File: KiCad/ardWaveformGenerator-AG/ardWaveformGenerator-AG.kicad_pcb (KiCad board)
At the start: 2 copper layers, 97.8 x 55.9 mm, 40 parts, among them SW1 SW_Rotary1x4, U1 Power in, U2 LM386, U3 Output

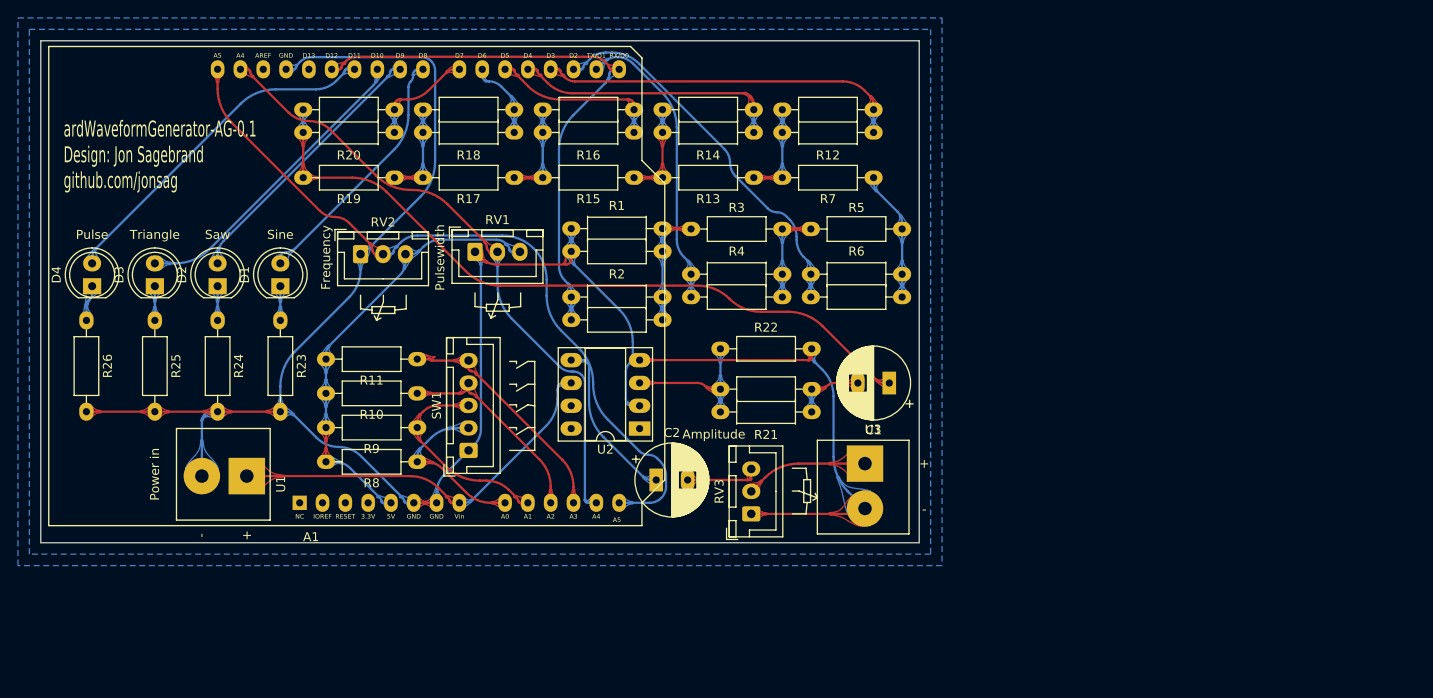
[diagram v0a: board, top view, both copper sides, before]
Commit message: ardWaveformGenerator-AG-pio with pcb-0.2
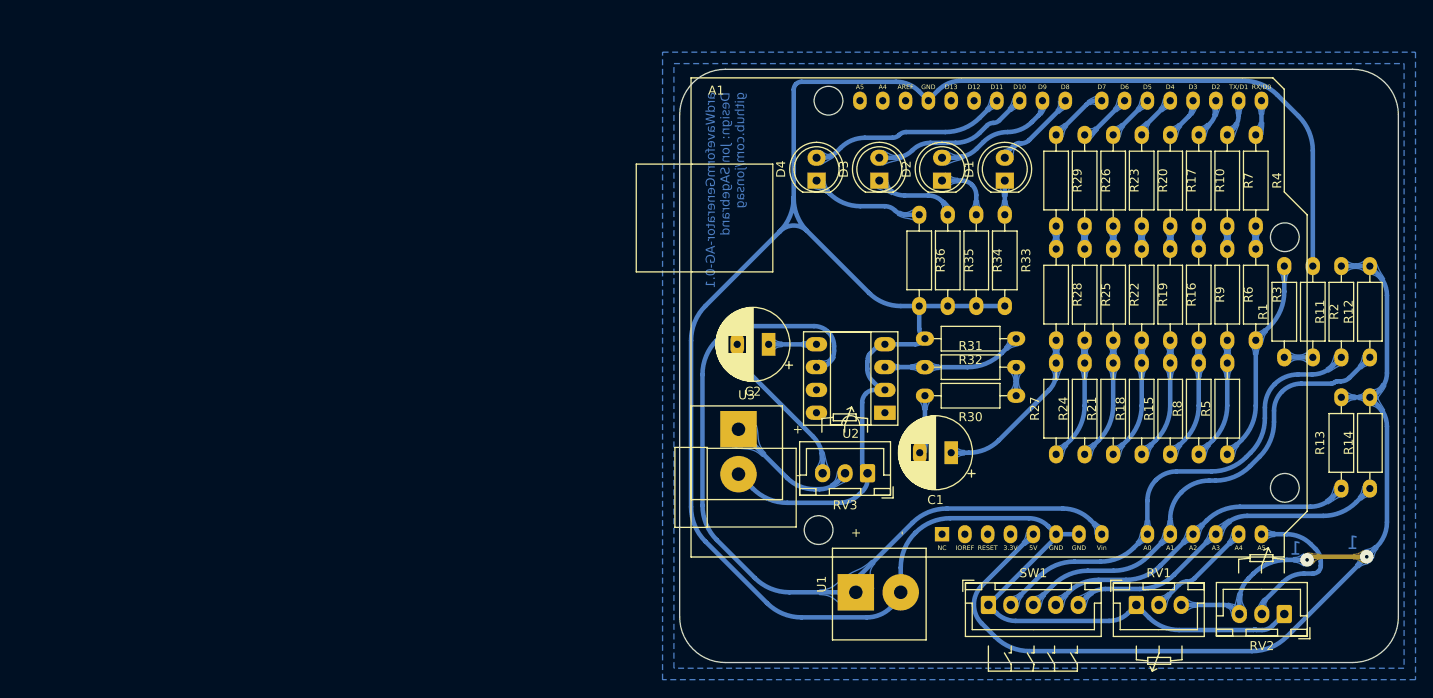
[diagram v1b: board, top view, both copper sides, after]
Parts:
- added R27: 10k, My_Misc:R_Axial_DIN0207_L6.3mm_D2.5mm_P10.16mm_Horizontal_large, F.Cu at (154.9, 107.6)
- added R28: 10k, My_Misc:R_Axial_DIN0207_L6.3mm_D2.5mm_P10.16mm_Horizontal_large, F.Cu at (154.9, 84.8)
- added R29: 10k, My_Misc:R_Axial_DIN0207_L6.3mm_D2.5mm_P10.16mm_Horizontal_large, F.Cu at (154.9, 72.1)
- added R30: 10k, My_Misc:R_Axial_DIN0207_L6.3mm_D2.5mm_P10.16mm_Horizontal_large, F.Cu at (150.5, 101.1)
- added R31: 10k, My_Misc:R_Axial_DIN0207_L6.3mm_D2.5mm_P10.16mm_Horizontal_large, F.Cu at (140.3, 97.9)
- added R32: 2.2k, My_Misc:R_Axial_DIN0207_L6.3mm_D2.5mm_P10.16mm_Horizontal_large, F.Cu at (150.5, 94.8)
- added R33: 220R, My_Misc:R_Axial_DIN0207_L6.3mm_D2.5mm_P10.16mm_Horizontal_large, F.Cu at (149.2, 81.0)
- added R34: 220R, My_Misc:R_Axial_DIN0207_L6.3mm_D2.5mm_P10.16mm_Horizontal_large, F.Cu at (146.1, 81.0)
- added R35: 220R, My_Misc:R_Axial_DIN0207_L6.3mm_D2.5mm_P10.16mm_Horizontal_large, F.Cu at (142.9, 81.0)
- added R36: 220R, My_Misc:R_Axial_DIN0207_L6.3mm_D2.5mm_P10.16mm_Horizontal_large, F.Cu at (139.7, 81.0)
- R1, R12, R14, R16, R18, R2, R20, R21, R4, R6: value 20k -> 10k; footprint My_Parts:R_Axial_parallell_DIN0207_L6.3mm_D2.5mm_P10.16mm_Horizontal_large -> My_Misc:R_Axial_DIN0207_L6.3mm_D2.5mm_P10.16mm_Horizontal_large
- R22: value 2.2k -> 10k
- R23, R24, R25, R26: value 220R -> 10k
- moved R26 113.0 mm to (158.1, 72.1)
- moved RV2 110.4 mm to (180.3, 125.4), turned to 180 degrees
- moved R25 103.8 mm to (158.1, 84.8)
- moved R11 102.9 mm to (186.7, 96.8), turned to 90 degrees
- moved R24 97.7 mm to (158.1, 107.6), turned to 90 degrees
- moved R23 95.0 mm to (161.3, 72.1)
- moved R10 91.6 mm to (170.8, 72.1), turned to -90 degrees
- moved R9 89.2 mm to (170.8, 84.8), turned to -90 degrees
- moved R8 87.0 mm to (170.8, 107.6), turned to 90 degrees
- moved R19 83.6 mm to (164.5, 84.8), turned to -90 degrees
- moved RV1 83.5 mm to (163.9, 124.4)
- moved R20 83.2 mm to (164.5, 72.1), turned to -90 degrees
- moved R2 82.8 mm to (183.5, 86.7), turned to -90 degrees
- moved D2 81.5 mm to (142.2, 77.2)
- moved D4 81.5 mm to (128.3, 77.2)
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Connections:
- A1 pad 27: D0 -> D12
- A1 pad 31: A4 -> unconnected-(A1-Pad31)
- A1 pad 32: A5 -> unconnected-(A1-Pad32)
- R1 pad 1: GND -> Net-(R1-Pad1)
- R1 pad 2: Net-(R1-Pad2) -> Net-(R5-Pad1)
- R10 pad 1: A2 -> D2
- R10 pad 2: +5V -> Net-(R10-Pad2)
- R11 pad 1: A3 -> A0
- R12 pad 1: D3 -> A1
- R12 pad 2: Net-(R12-Pad2) -> +5V
- R13 pad 1: Net-(R12-Pad2) -> A2
- R13 pad 2: Net-(R13-Pad2) -> +5V
- R14 pad 1: D4 -> A3
- R14 pad 2: Net-(R13-Pad2) -> +5V
- R15 pad 1: Net-(R13-Pad2) -> Net-(R8-Pad2)
- R15 pad 2: Net-(R15-Pad2) -> Net-(R18-Pad1)
- R16 pad 1: D5 -> Net-(R16-Pad1)
- R16 pad 2: Net-(R15-Pad2) -> Net-(R18-Pad1)
- R17 pad 1: Net-(R15-Pad2) -> D3
- R17 pad 2: Net-(R17-Pad2) -> Net-(R16-Pad1)
- R18 pad 1: D6 -> Net-(R18-Pad1)
- R18 pad 2: Net-(R17-Pad2) -> Net-(R18-Pad2)
- R19 pad 1: Net-(R17-Pad2) -> Net-(R19-Pad1)
- R19 pad 2: Net-(C1-Pad1) -> Net-(R18-Pad2)
- R2 pad 1: D0 -> GND
- R2 pad 2: Net-(R1-Pad2) -> Net-(R1-Pad1)
- R20 pad 1: D7 -> D4
- R20 pad 2: Net-(C1-Pad1) -> Net-(R19-Pad1)
- R21 pad 1: Net-(C1-Pad2) -> Net-(R18-Pad2)
- R22 pad 1: Net-(R21-Pad2) -> Net-(R22-Pad1)
- R22 pad 2: GND -> Net-(R21-Pad2)
- R23 pad 1: Net-(D1-Pad1) -> D5
- R23 pad 2: GND -> Net-(R22-Pad1)
- R24 pad 1: Net-(D2-Pad1) -> Net-(R21-Pad2)
- R24 pad 2: GND -> Net-(R24-Pad2)
- R25 pad 1: Net-(D3-Pad1) -> Net-(R25-Pad1)
- R25 pad 2: GND -> Net-(R24-Pad2)
- R26 pad 1: Net-(D4-Pad1) -> D6
- R26 pad 2: GND -> Net-(R25-Pad1)
- R3 pad 1: Net-(R1-Pad2) -> Net-(R3-Pad1)
- R3 pad 2: Net-(R3-Pad2) -> Net-(R5-Pad1)
- R4 pad 1: D1 -> D0
- R4 pad 2: Net-(R3-Pad2) -> Net-(R3-Pad1)
- R5 pad 1: Net-(R3-Pad2) -> Net-(R5-Pad1)
- R6 pad 1: D2 -> Net-(R6-Pad1)
- R7 pad 1: Net-(R5-Pad2) -> D1
- R7 pad 2: Net-(R12-Pad2) -> Net-(R6-Pad1)
- R8 pad 1: A0 -> Net-(R5-Pad2)
- R8 pad 2: +5V -> Net-(R8-Pad2)
- R9 pad 1: A1 -> Net-(R10-Pad2)
- R9 pad 2: +5V -> Net-(R8-Pad2)
- U2 pad 3: Net-(R21-Pad2) -> Net-(R31-Pad1)
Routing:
- net +5V: track 49.6 -> 126.4 mm, vias 0 -> 2
- net GND: track 234.4 -> 307.5 mm
- net A5: track 85.6 -> 17.9 mm
- net Net-(C1-Pad1): track 81.0 -> 19.3 mm
- net D0: track 64.3 -> 4.02 mm
- net A4: track 70.1 -> 12.0 mm
- net VCC: track 44.2 -> 91.4 mm
- net D2: track 42.3 -> 4.49 mm
- net D3: track 40.8 -> 4.79 mm
- net A0: track 19.1 -> 52.2 mm
- net D1: track 32.9 -> 4.23 mm
- net A1: track 23.3 -> 51.8 mm
- net D4: track 30.0 -> 5.09 mm
- net Net-(R5-Pad1): track 0.00 -> 23.1 mm
- net D8: track 28.6 -> 9.61 mm
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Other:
- board size 97.8 x 55.9 mm -> 80 x 66 mm
- board text added: "${TITLE}-${REVISION} Design: Jon SAgebrand github.com/jonsag"
- board text added: "1"
- board text removed: "${TITLE}-${REVISION} Design: Jon Sagebrand github.com/jonsag"
- board text removed: "Amplitude"
- board text removed: "Frequency"
- board text removed: "Power in"
- board text removed: "Pulse"
- board text removed: "Pulsewidth"
- board text removed: "Saw"
- board text removed: "Sine"
- board text removed: "Triangle"
